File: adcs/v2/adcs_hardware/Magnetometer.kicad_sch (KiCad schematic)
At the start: 1 part, among them U3 LIS2MDL

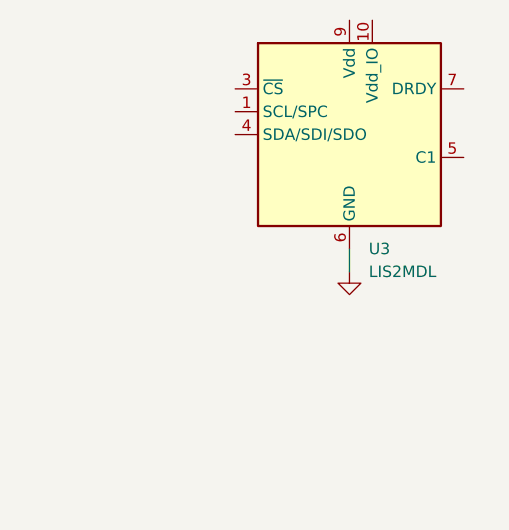
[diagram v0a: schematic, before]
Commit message: magnetometer subsheet wiring
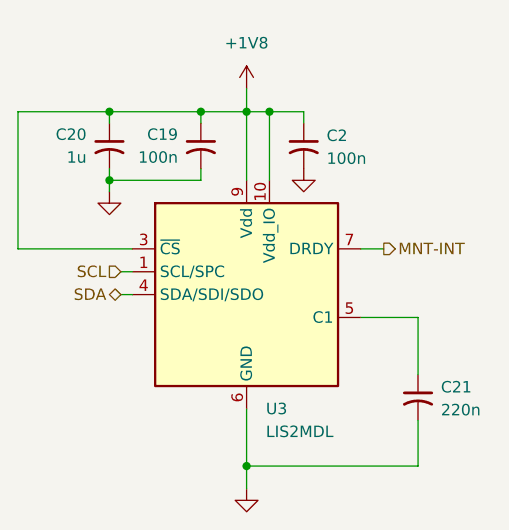
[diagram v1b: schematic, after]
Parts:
- added C19, C2: 100n, Package_DIP:DIP-8_W7.62mm, symbol Device:C_Small_US
- added C20: 1u, Package_DIP:DIP-8_W7.62mm, symbol Device:C_Small_US
- added C21: 220n, Package_DIP:DIP-8_W7.62mm, symbol Device:C_Small_US
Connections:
- net GND: now also C19.2, C2.2, C20.2, C21.2
- net SCL: now reaches U3.1 (SCL/SPC)
- net +1V8: now reaches U3.10 (Vdd_IO)
- net +1V8: now also U3.3 (~{CS}), U3.9 (Vdd), C19.1, C2.1, C20.1
- net SDA: now reaches U3.4 (SDA/SDI/SDO)
- net at U3.5 (C1): now also C21.1
- net MNT-INT: now reaches U3.7 (DRDY)
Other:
- moved on the sheet: U3
